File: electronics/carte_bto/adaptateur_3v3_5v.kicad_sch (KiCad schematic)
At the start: 40 parts, among them Q1 MMBT2222A, Q2 MMBT2222A, Q3 MMBT2222A, Q4 MMBT2222A, Q5 MMBT2222A, Q6 MMBT2222A, Q7 MMBT2222A, Q8 MMBT2222A

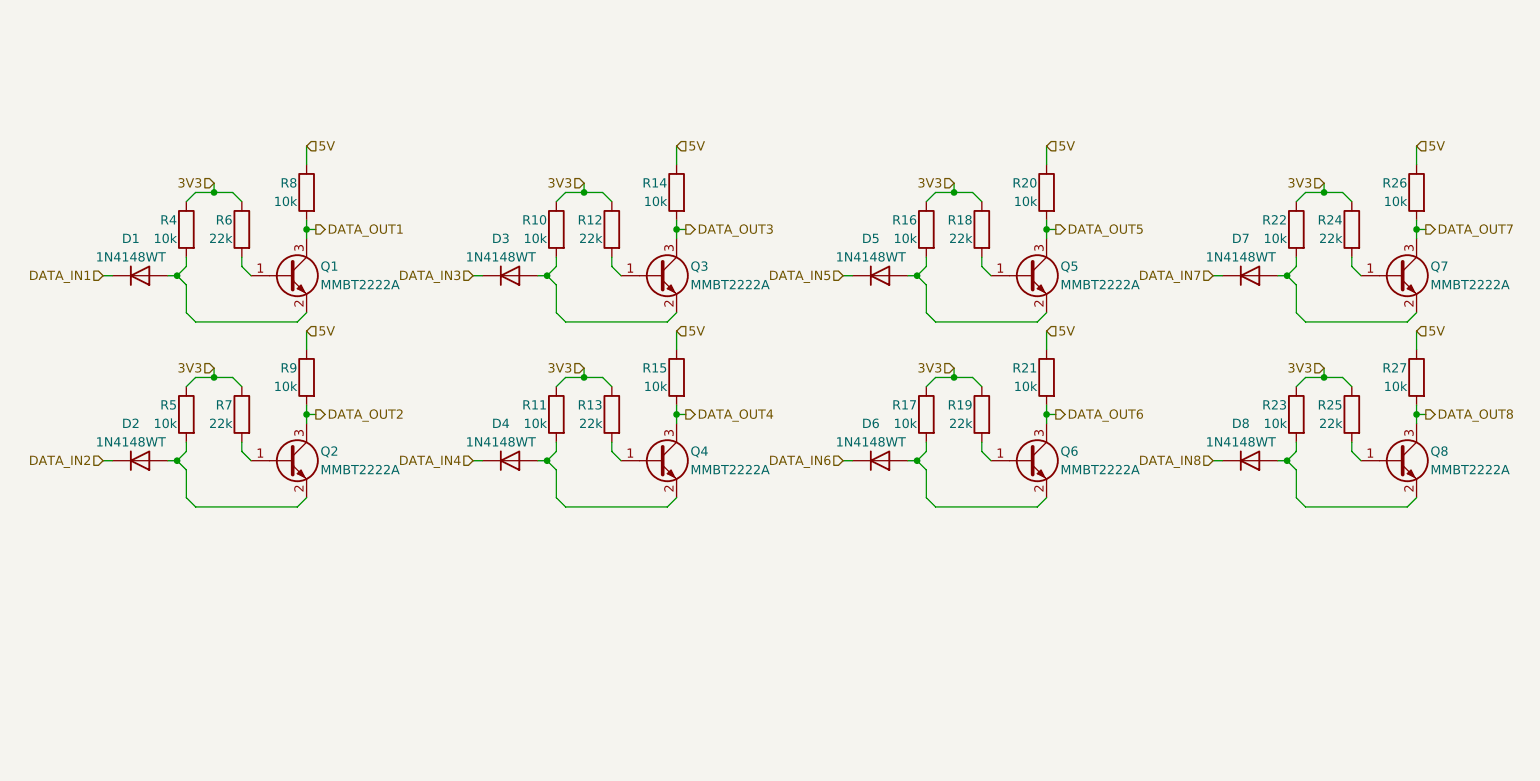
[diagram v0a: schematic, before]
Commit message: BTO schematic: cleanup and documentation
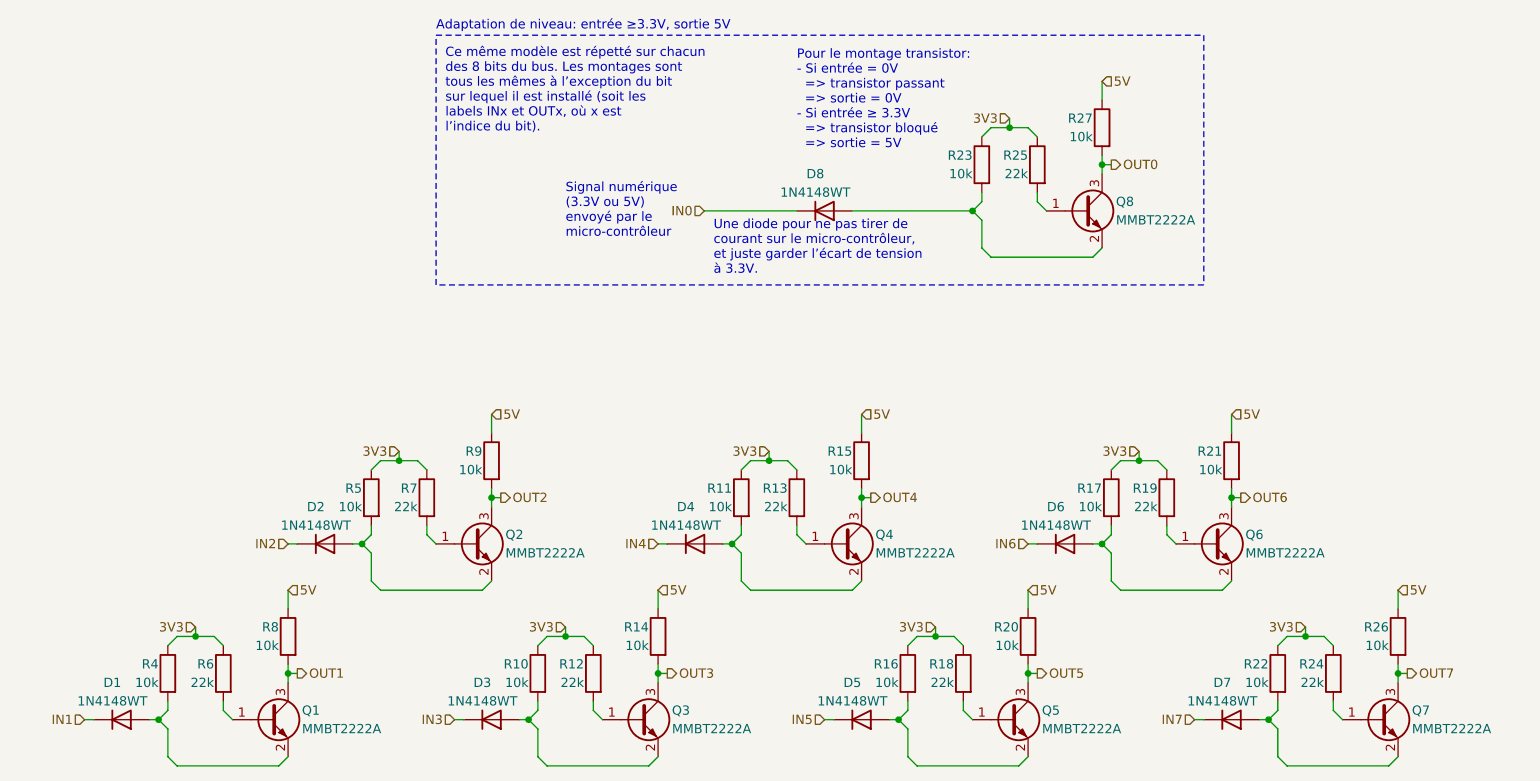
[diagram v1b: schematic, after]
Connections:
- net DATA_IN1 renamed IN1
- net DATA_IN2 renamed IN2
- net DATA_IN3 renamed IN3
- net DATA_IN4 renamed IN4
- net DATA_IN5 renamed IN5
- net DATA_IN6 renamed IN6
- net DATA_IN7 renamed IN7
- net DATA_IN8 renamed IN0
- net DATA_OUT1 renamed OUT1
- net DATA_OUT2 renamed OUT2
- net DATA_OUT3 renamed OUT3
- net DATA_OUT4 renamed OUT4
- net DATA_OUT5 renamed OUT5
- net DATA_OUT6 renamed OUT6
- net DATA_OUT7 renamed OUT7
- net DATA_OUT8 renamed OUT0
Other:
- note added: "Adaptation de niveau: entrée ≥3.3V, sortie 5V"
- note added: "Ce même modèle est répetté sur chacun des 8 bits du bus. Les montages sont tous les mêmes à l’exception du bit sur lequel il est installé (soit les labels INx et OUTx, où x est l’indice du bit)."
- note added: "Pour le montage transistor: - Si entrée = 0V => transistor passant => sortie = 0V - Si entrée ≥ 3.3V => transistor bloqué => sortie = 5V"
- note added: "Signal numérique (3.3V ou 5V) envoyé par le micro-contrôleur"
- note added: "Une diode pour ne pas tirer de courant sur le micro-contrôleur, et juste garder l’écart de tension à 3.3V."
- moved on the sheet: D1, D2, D3, D4, D5, D6, D7, D8, Q1, Q2, Q3, Q4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
